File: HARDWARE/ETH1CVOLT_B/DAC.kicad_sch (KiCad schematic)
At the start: 37 parts, among them J1 Conn_Coaxial, U1 ADG5419BRMZ-RL7, U2 ADA4522-4ARUZ, U3 DAC81401PWR, U4 DAC81401PWR, U5 ADA4522-1ARMZ

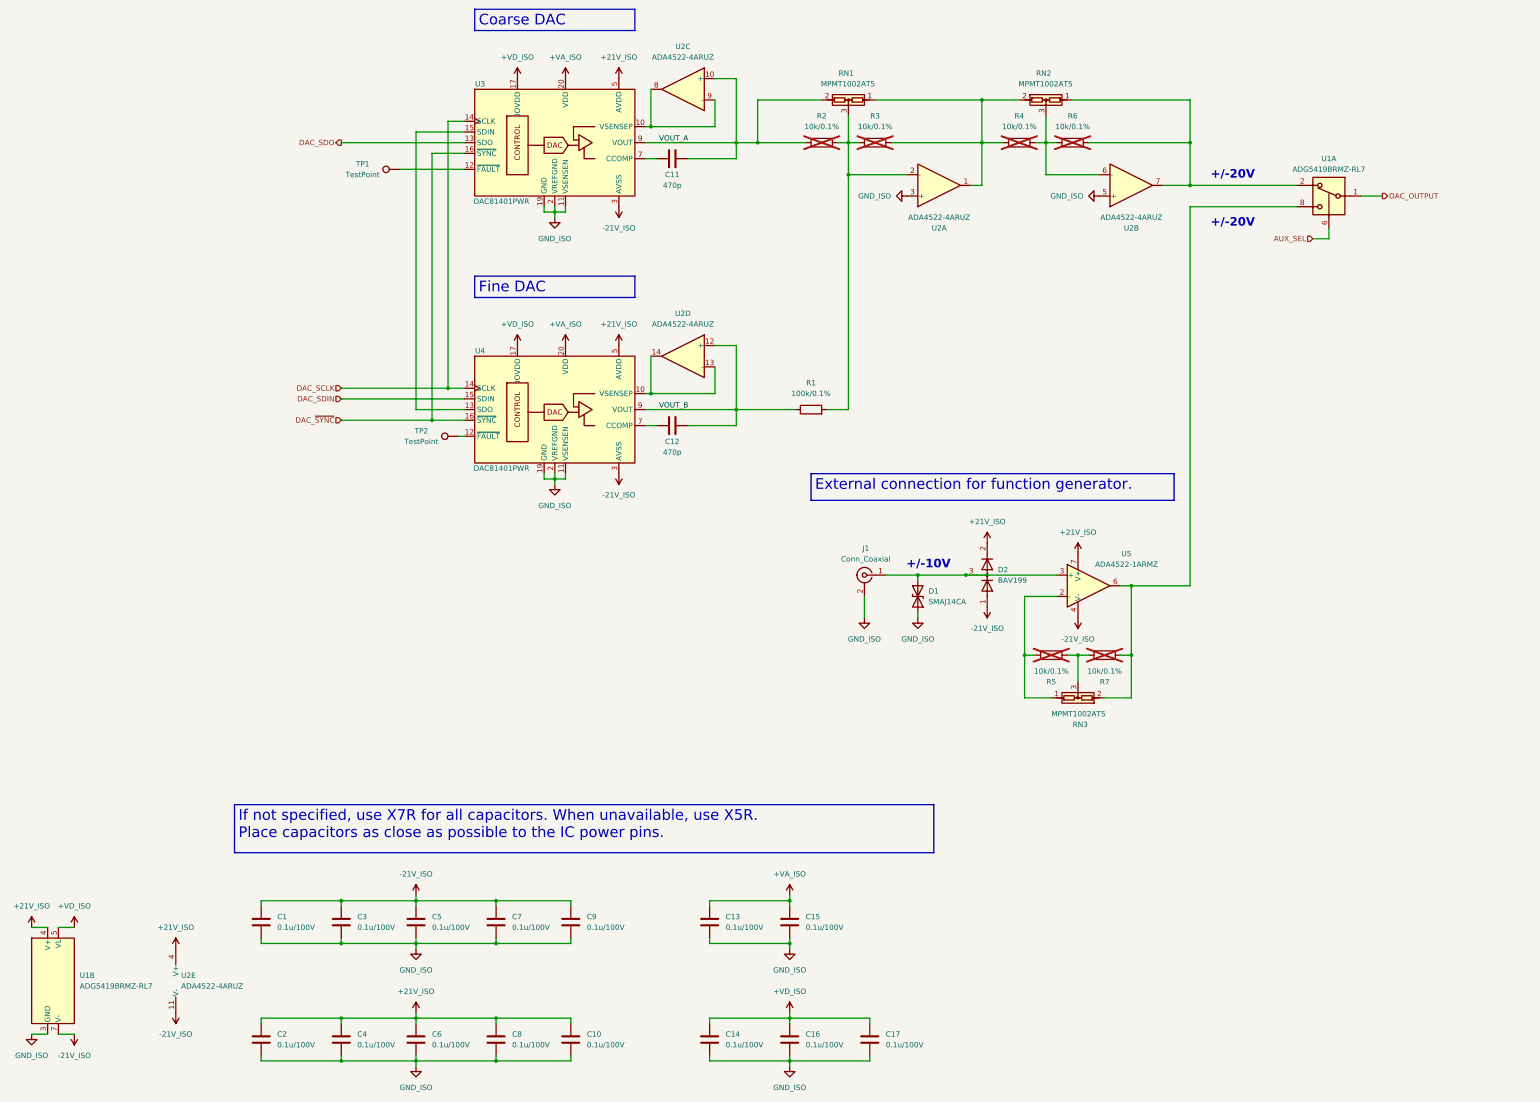
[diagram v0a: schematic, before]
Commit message: Development
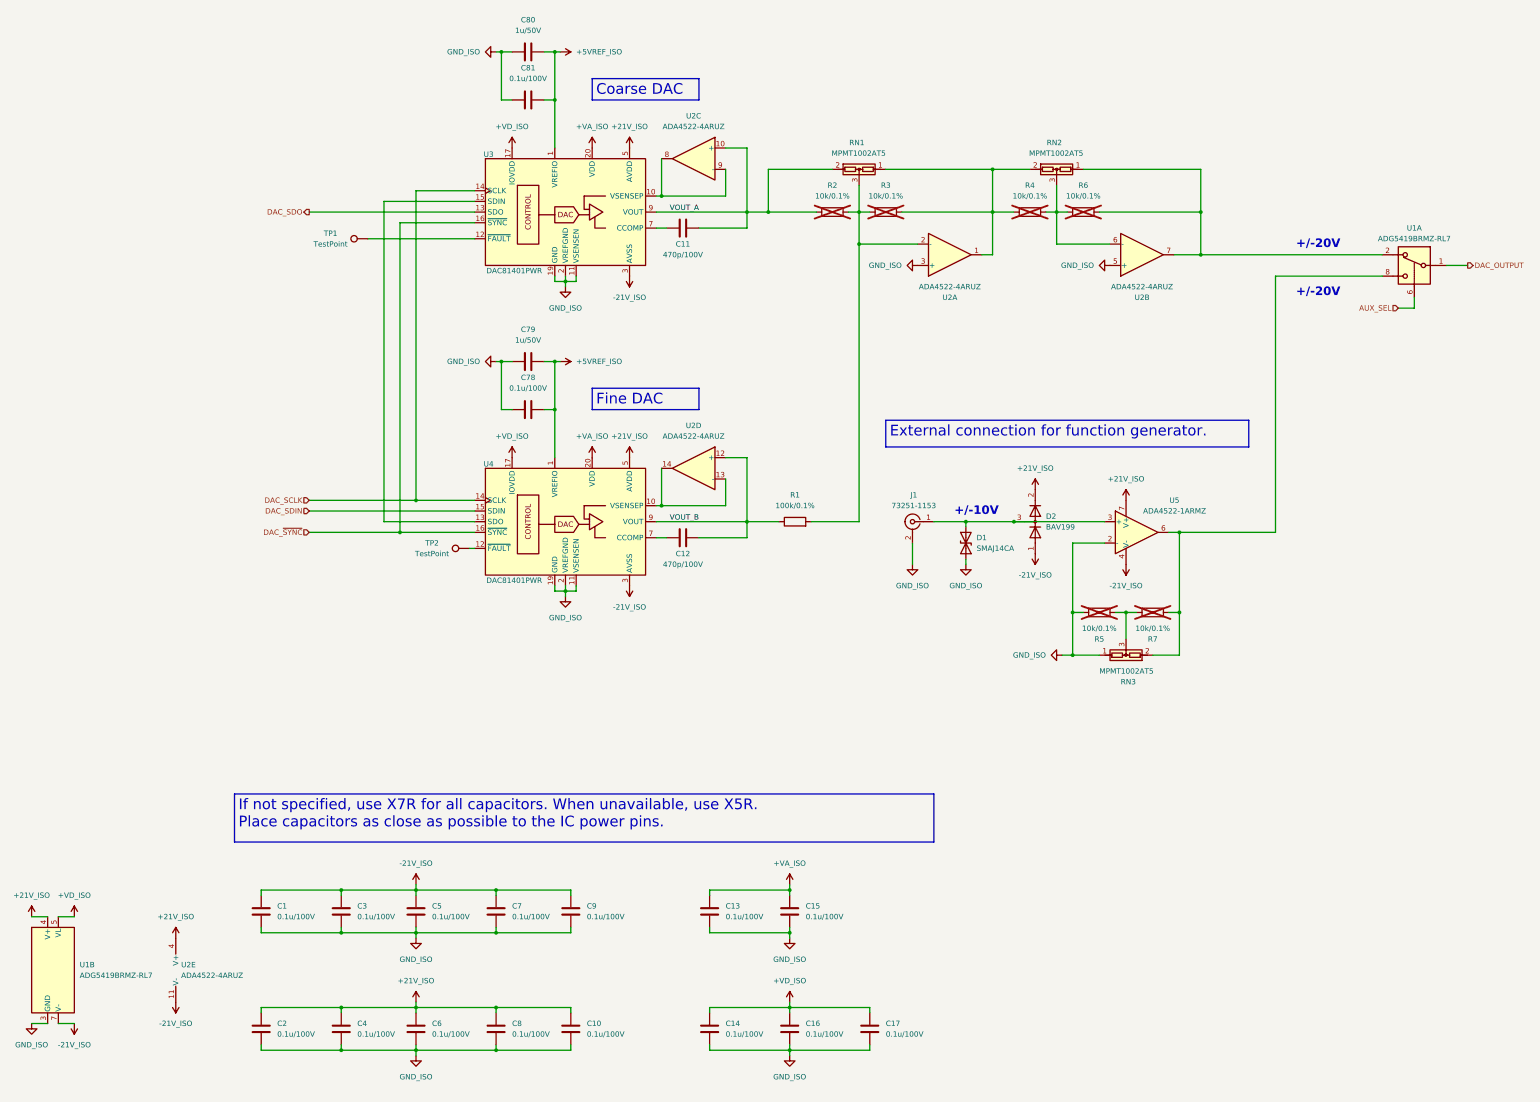
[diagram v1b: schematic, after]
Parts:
- added C78, C81: 0.1u/100V, Capacitor_SMD:C_0603_1608Metric_Pad1.08x0.95mm_HandSolder, symbol Device:C
- added C79, C80: 1u/50V, Capacitor_SMD:C_0603_1608Metric_Pad1.08x0.95mm_HandSolder, symbol Device:C
- C1, C10, C13, C14, C15, C16, C17, C2, C3, C4, C5, C6, C7, C8, C9: footprint (none) -> Capacitor_SMD:C_0603_1608Metric_Pad1.08x0.95mm_HandSolder
- C11, C12: value 470p -> 470p/100V
- J1: value Conn_Coaxial -> 73251-1153; footprint (none) -> Connector_Coaxial:SMA_Molex_73251-1153_EdgeMount_Horizontal
- TP1, TP2: footprint (none) -> TestPoint:TestPoint_Pad_D1.5mm; now left out of the parts list
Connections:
- net GND_ISO: now also R5.2, RN3.1, U5.2 (-), C78.1, C79.1, C80.1, C81.1
- new net +5VREF_ISO: C78.2, C79.2, C80.2, C81.2, U3.1 (VREFIO), U4.1 (VREFIO)
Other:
- moved on the sheet: C1, C10, C11, C12, C13, C14, C15, C16, C17, C2, C3, C4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
